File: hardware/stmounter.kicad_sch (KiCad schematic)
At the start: 13 parts, among them J1 USB_C_Receptacle_USB2.0_14P, J2 Conn_01x20, J3 Conn_01x20, SW1 SW_Push, U1 STM32F103C8Tx, U2 SRV05-4, U3 AMS1117-3.3

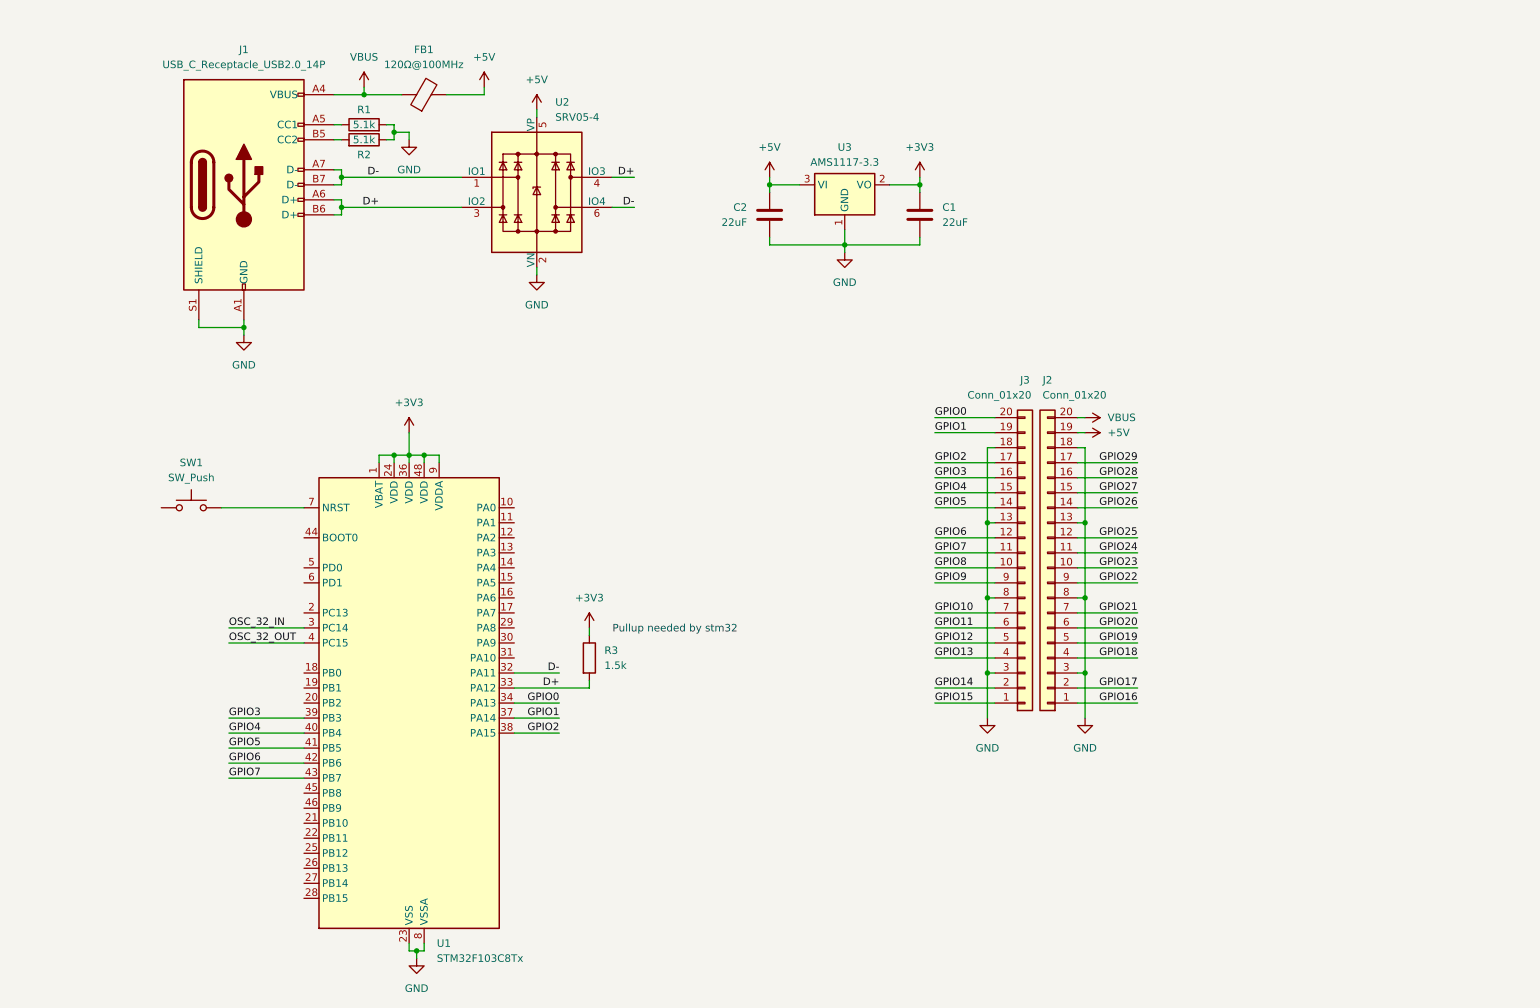
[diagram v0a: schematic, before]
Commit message: Progress
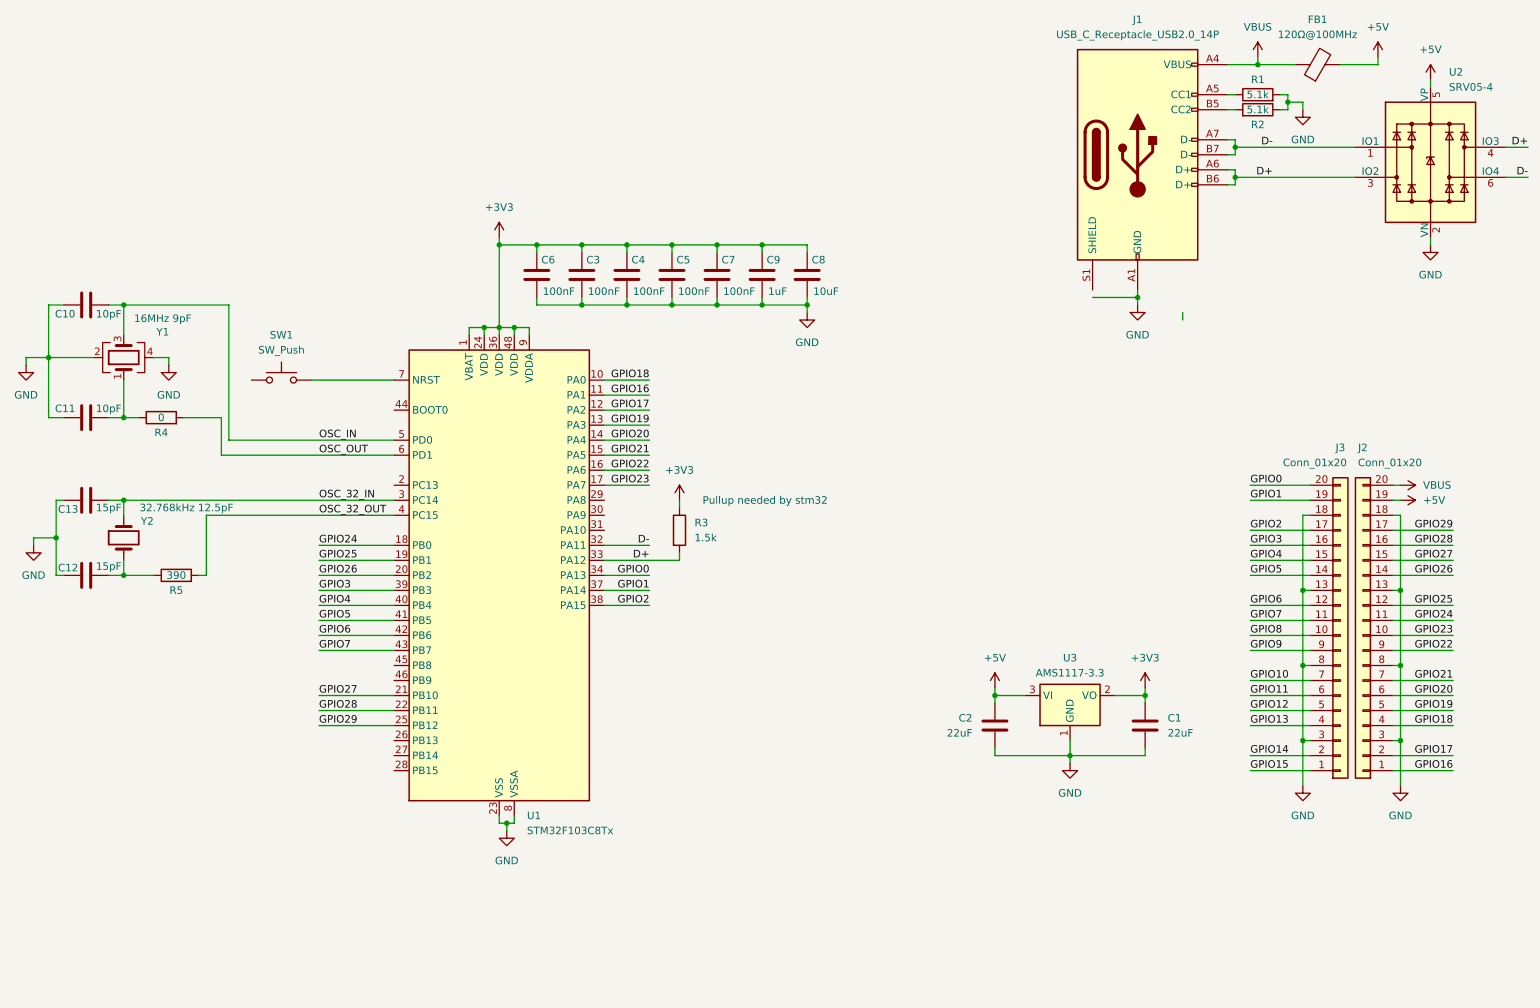
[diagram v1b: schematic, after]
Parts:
- added C10, C11: 10pF, Capacitor_SMD:C_0402_1005Metric, symbol Device:C
- added C12, C13: 15pF, Capacitor_SMD:C_0402_1005Metric, symbol Device:C
- added C3, C4, C5, C6, C7: 100nF, Capacitor_SMD:C_0402_1005Metric, symbol Device:C
- added C8: 10uF, Capacitor_SMD:C_0402_1005Metric, symbol Device:C
- added C9: 1uF, Capacitor_SMD:C_0402_1005Metric, symbol Device:C
- added R4: 0, Resistor_SMD:R_0402_1005Metric, symbol Device:R
- added R5: 390, Resistor_SMD:R_0402_1005Metric, symbol Device:R
- added Y1: 16MHz 9pF, Crystal:Crystal_SMD_3225-4Pin_3.2x2.5mm, symbol Device:Crystal_GND24
- added Y2: 32.768kHz 12.5pF, Crystal:Crystal_SMD_3215-2Pin_3.2x1.5mm, symbol Device:Crystal
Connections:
- net +3V3: now also C3.1, C4.1, C5.1, C6.1, C7.1, C8.1, C9.1
- net GND: now also C10.1, C11.1, C12.1, C13.1, C3.2, C4.2, C5.2, C6.2, C7.2, C8.2, C9.2, Y1.2, Y1.4; no longer J1.S1 (SHIELD)
- net GPIO16: now also U1.11 (PA1)
- net GPIO17: now also U1.12 (PA2)
- net GPIO18: now also U1.10 (PA0)
- net GPIO19: now also U1.13 (PA3)
- net GPIO20: now also U1.14 (PA4)
- net GPIO21: now also U1.15 (PA5)
- net GPIO22: now also U1.16 (PA6)
- net GPIO23: now also U1.17 (PA7)
- net GPIO24: now also U1.18 (PB0)
- net GPIO25: now also U1.19 (PB1)
- net GPIO26: now also U1.20 (PB2)
- net GPIO27: now also U1.21 (PB10)
- net GPIO28: now also U1.22 (PB11)
- net GPIO29: now also U1.25 (PB12)
- net OSC_32_IN: now also C13.2, Y2.1
- net OSC_32_OUT: now also R5.2
- net OSC_IN: now reaches U1.5 (PD0)
- net OSC_IN: now also C10.2, Y1.3
- net OSC_OUT: now reaches U1.6 (PD1)
- net OSC_OUT: now also R4.2
- new net: C11.2, R4.1, Y1.1
- new net: C12.2, R5.1, Y2.2
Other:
- moved on the sheet: C1, C2, FB1, J1, J2, J3, R1, R2, R3, SW1, U1, U2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
